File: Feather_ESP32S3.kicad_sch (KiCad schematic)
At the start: 15 parts, among them J1 Conn_01x02, Q1 AO3401A, SW1 SW_Push, U1 ESP32-S3-MINI-1, U2 LGS4056H, U3 RT9013-xxGB

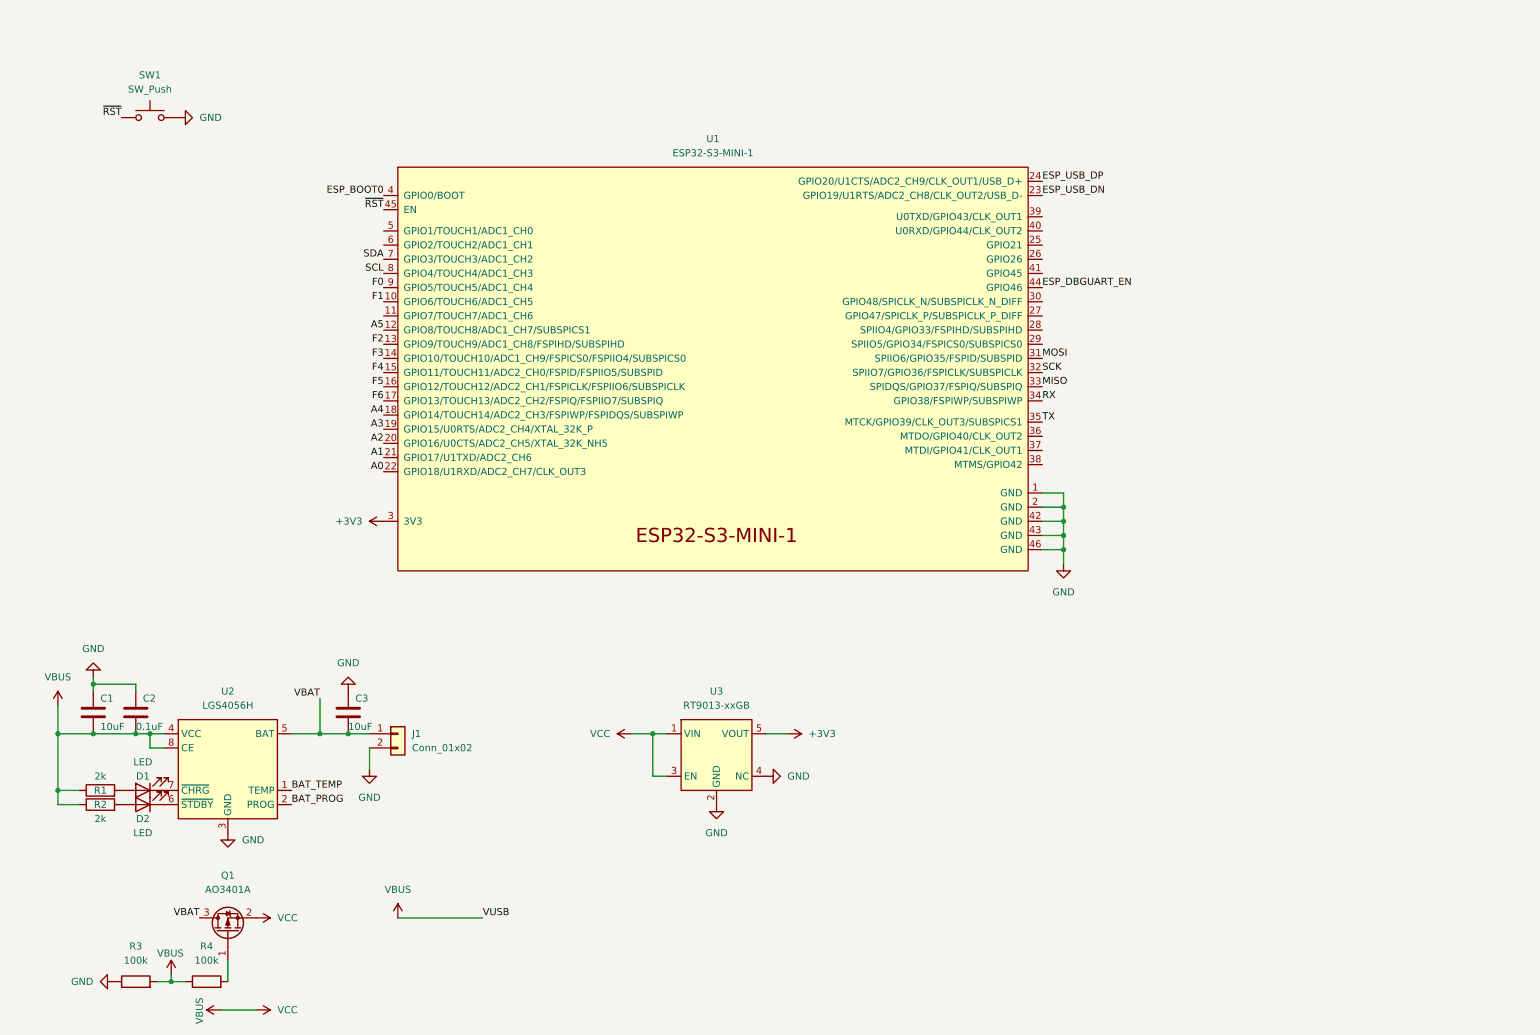
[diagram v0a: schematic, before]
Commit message: Latest HW
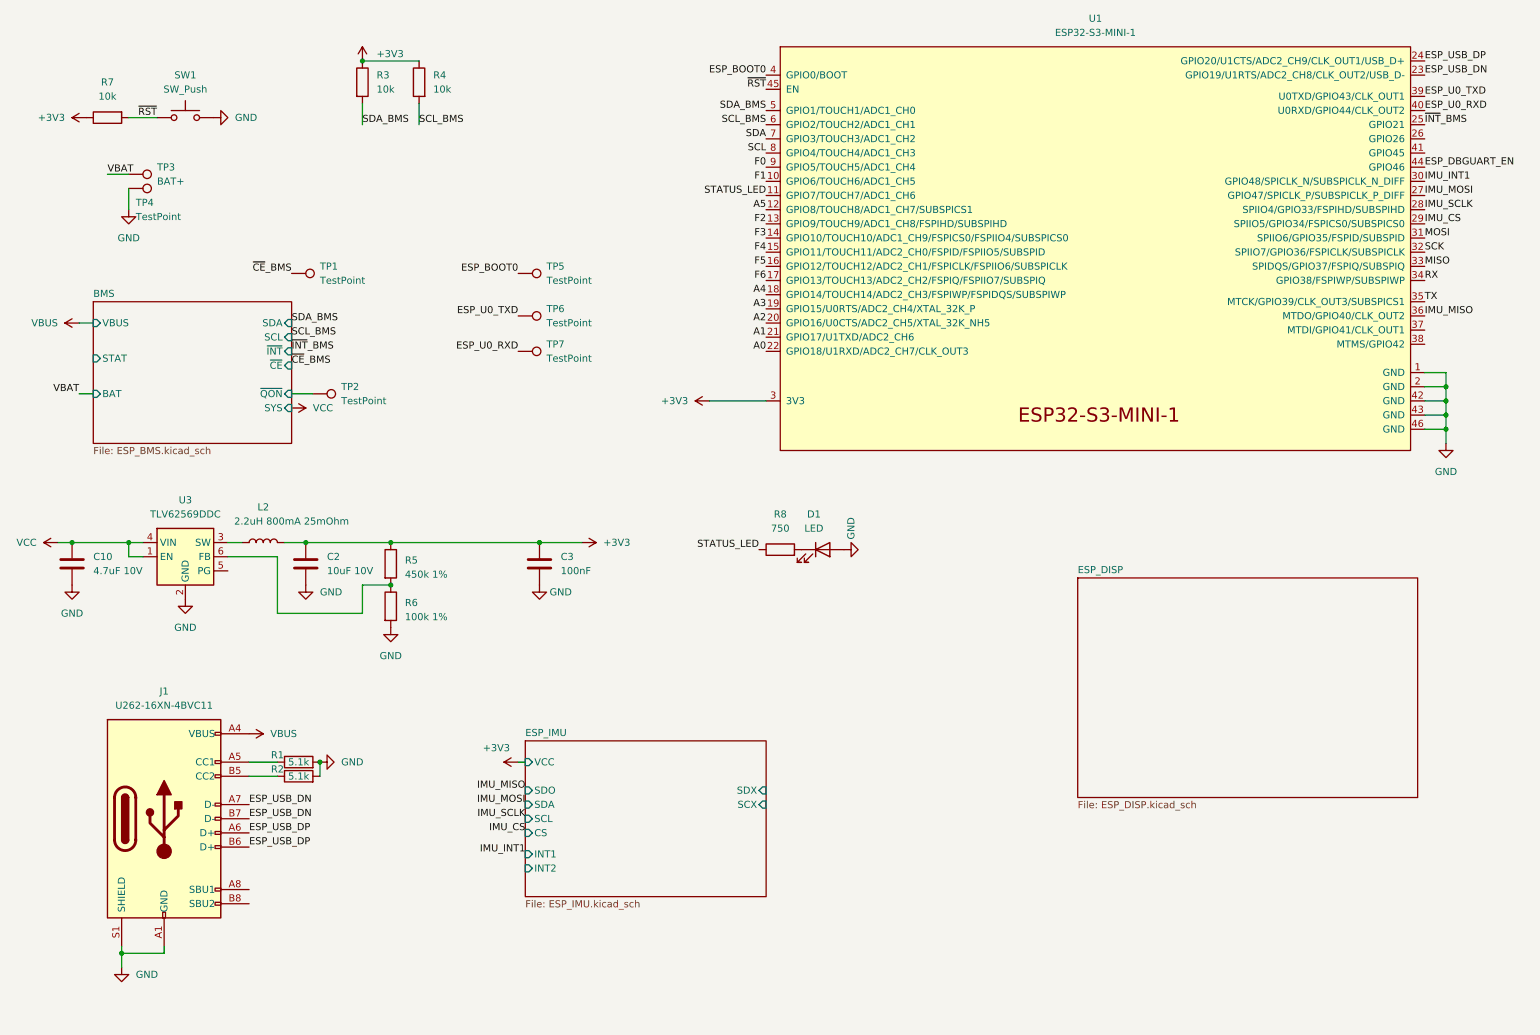
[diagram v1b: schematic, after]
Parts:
- removed C1: 10uF, Capacitor_SMD:C_0603_1608Metric, symbol Device:C
- removed D2: LED, LED_SMD:LED_0402_1005Metric, symbol Device:LED
- removed J1: Conn_01x02, Connector_JST:JST_PH_S2B-PH-SM4-TB_1x02-1MP_P2.00mm_Horizontal, symbol Connector_Generic:Conn_01x02
- removed Q1: AO3401A, Package_TO_SOT_SMD:SOT-23, symbol Transistor_FET:AO3401A
- removed U2: LGS4056H, Package_DFN_QFN:DFN-8-1EP_2x2mm_P0.5mm_EP0.9x1.5mm, symbol Power_Management:TP4056
- removed U3: RT9013-xxGB, Package_TO_SOT_SMD:SOT-23-5, symbol Regulator_Linear:RT9013-xxGB
- added C10: 4.7uF 10V, Capacitor_SMD:C_0402_1005Metric, symbol Device:C
- added J1: U262-16XN-4BVC11, Connector_USB:USB_C_Receptacle_XKB_U262-16XN-4BVC11, symbol Connector:USB_C_Receptacle_USB2.0
- added L2: 2.2uH 800mA 25mOhm, Inductor_SMD:L_0805_2012Metric, symbol Device:L
- added R5: 450k 1%, Resistor_SMD:R_0402_1005Metric, symbol Device:R
- added R6: 100k 1%, Resistor_SMD:R_0402_1005Metric, symbol Device:R
- added R7: 10k, Resistor_SMD:R_0402_1005Metric, symbol Device:R
- added R8: 750, Resistor_SMD:R_0402_1005Metric, symbol Device:R
- added TP1, TP2, TP4, TP5, TP6, TP7: TestPoint, TestPoint:TestPoint_Pad_D1.0mm, symbol Connector:TestPoint
- added TP3: BAT+, TestPoint:TestPoint_Pad_D1.0mm, symbol Connector:TestPoint
- added U3: TLV62569DDC, Package_TO_SOT_SMD:SOT-23-6, symbol Regulator_Switching:TLV62569DDC
- C2: value 0.1uF -> 10uF 10V; footprint Capacitor_SMD:C_0603_1608Metric -> Capacitor_SMD:C_0402_1005Metric
- C3: value 10uF -> 100nF; footprint Capacitor_SMD:C_0603_1608Metric -> Capacitor_SMD:C_0402_1005Metric
- R1, R2: value 2k -> 5.1k
- R3, R4: value 100k -> 10k; footprint (none) -> Resistor_SMD:R_0402_1005Metric
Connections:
- net +3V3: now also C2.1, C3.1, R3.1, R4.1, L2.2, R5.1, R7.1
- net ESP_BOOT0: now also TP5.1
- net ESP_USB_DN: now also J1.A7 (D-), J1.B7 (D-)
- net ESP_USB_DP: now also J1.A6 (D+), J1.B6 (D+)
- net GND: now also C2.2, C3.2, D1.2 (A), R1.2, R2.2, C10.2, J1.A1 (GND), J1.A12 (GND), J1.B1 (GND), J1.B12 (GND), J1.S1 (SHIELD), R6.2, TP4.1, U3.2 (GND); no longer C2.1, C3.1, R3.1
- net VBAT: now also TP3.1; no longer C3.2
- net VBUS: now also J1.A4 (VBUS), J1.A9 (VBUS), J1.B4 (VBUS), J1.B9 (VBUS); no longer C2.2, R1.1, R2.1, R3.2, R4.1
- net ~{RST}: now also R7.2
- net SCL_BMS: now reaches R4.2
- net SCL_BMS: now also U1.6 (GPIO2/TOUCH2/ADC1_CH1)
- net STATUS_LED: now reaches U1.11 (GPIO7/TOUCH7/ADC1_CH6)
- net STATUS_LED: now also R8.1
- net ~{INT}_BMS: now reaches U1.25 (GPIO21)
- net IMU_MOSI: now reaches U1.27 (GPIO47/SPICLK_P/SUBSPICLK_P_DIFF)
- net IMU_SCLK: now reaches U1.28 (SPIIO4/GPIO33/FSPIHD/SUBSPIHD)
- net IMU_CS: now reaches U1.29 (SPIIO5/GPIO34/FSPICS0/SUBSPICS0)
- net IMU_INT1: now reaches U1.30 (GPIO48/SPICLK_N/SUBSPICLK_N_DIFF)
- net IMU_MISO: now reaches U1.36 (MTDO/GPIO40/CLK_OUT2)
- net ESP_U0_TXD: now reaches U1.39 (U0TXD/GPIO43/CLK_OUT1)
- net ESP_U0_TXD: now also TP6.1
- net ESP_U0_RXD: now reaches U1.40 (U0RXD/GPIO44/CLK_OUT2)
- net ESP_U0_RXD: now also TP7.1
- net SDA_BMS: now reaches U1.5 (GPIO1/TOUCH1/ADC1_CH0)
- net SDA_BMS: now also R3.2
- net at D1.1 (K): now also R8.2
- new net: L2.1, U3.3 (SW)
- new net: R5.2, R6.1, U3.6 (FB)
- new net: J1.A5 (CC1), R1.1
- new net: J1.B5 (CC2), R2.1
- new net BMS/~{QON}: TP2.1
- new net VCC: C10.1, U3.1 (EN), U3.4 (VIN)
- new net ~{CE}_BMS: TP1.1
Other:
- added sheet BMS (ESP_BMS.kicad_sch)
- added sheet ESP_DISP (ESP_DISP.kicad_sch)
- added sheet ESP_IMU (ESP_IMU.kicad_sch)
- moved on the sheet: SW1, U1
